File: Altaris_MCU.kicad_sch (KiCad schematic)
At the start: 89 parts, among them J1 Screw_Terminal_01x02, J10 USB_C_Receptacle_USB2.0_16P, J11 Screw_Terminal_01x02, J12 Screw_Terminal_01x02, J13 Screw_Terminal_01x02, J14 Screw_Terminal_01x02, J16 Conn_01x06, J2 Screw_Terminal_01x02, J3 Screw_Terminal_01x02, J4 Screw_Terminal_01x02, J5 Screw_Terminal_01x02, J6 Screw_Terminal_01x02, J7 Conn_01x08_Socket, J8 Screw_Terminal_01x02, J9 USB_C_Receptacle_USB2.0_16P, Q1 Q_NMOS, SW2 RESET1, SW3 BOOT1, U1 ESP32-S3-WROOM-1, U10 USBLC6-2SC6, U11 MAX31855TASA, U12 TPS62827DMQT, U13 USBLC6-2SC6, U15 CH340X, U17 MAX31855TASA, U18 MAX31855TASA, U2 MAX31855KASA, U3 TPS79333-EP, U4 ICM-20948, U5 TPS79318-EP, U6 SN74AVC4T774RSVR, U7 MAX31855KASA, U8 MAX31855KASA, U9 SN74AVC4T774RSVR

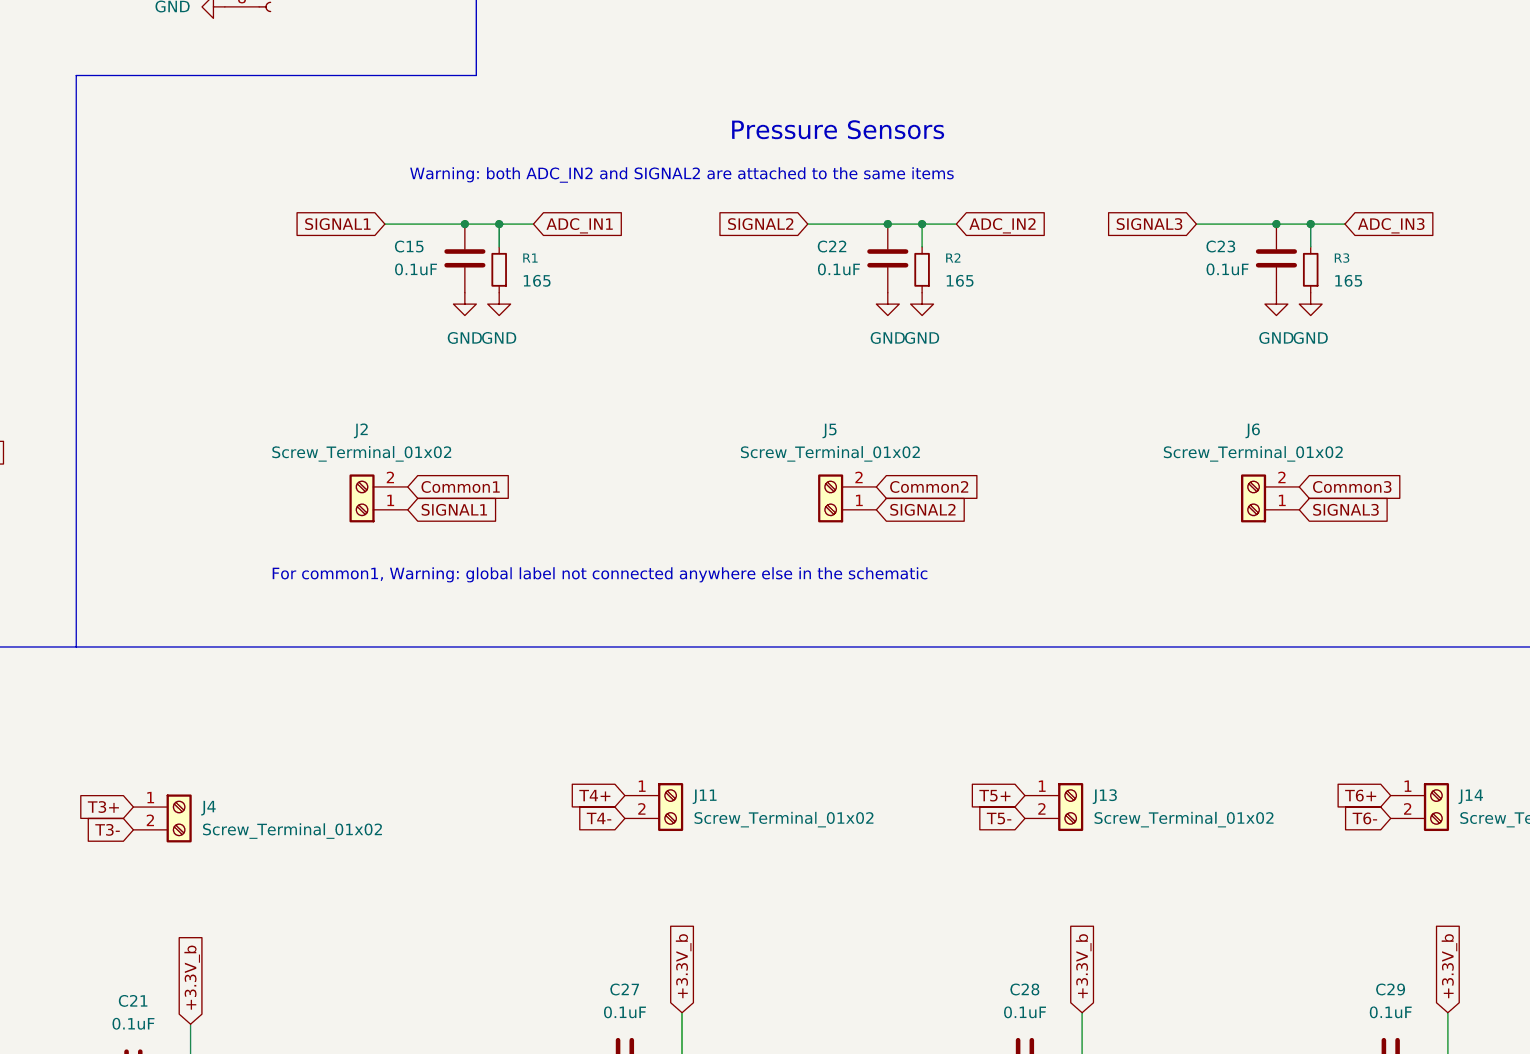
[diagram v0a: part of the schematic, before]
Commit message: minor edits to layout and schematic
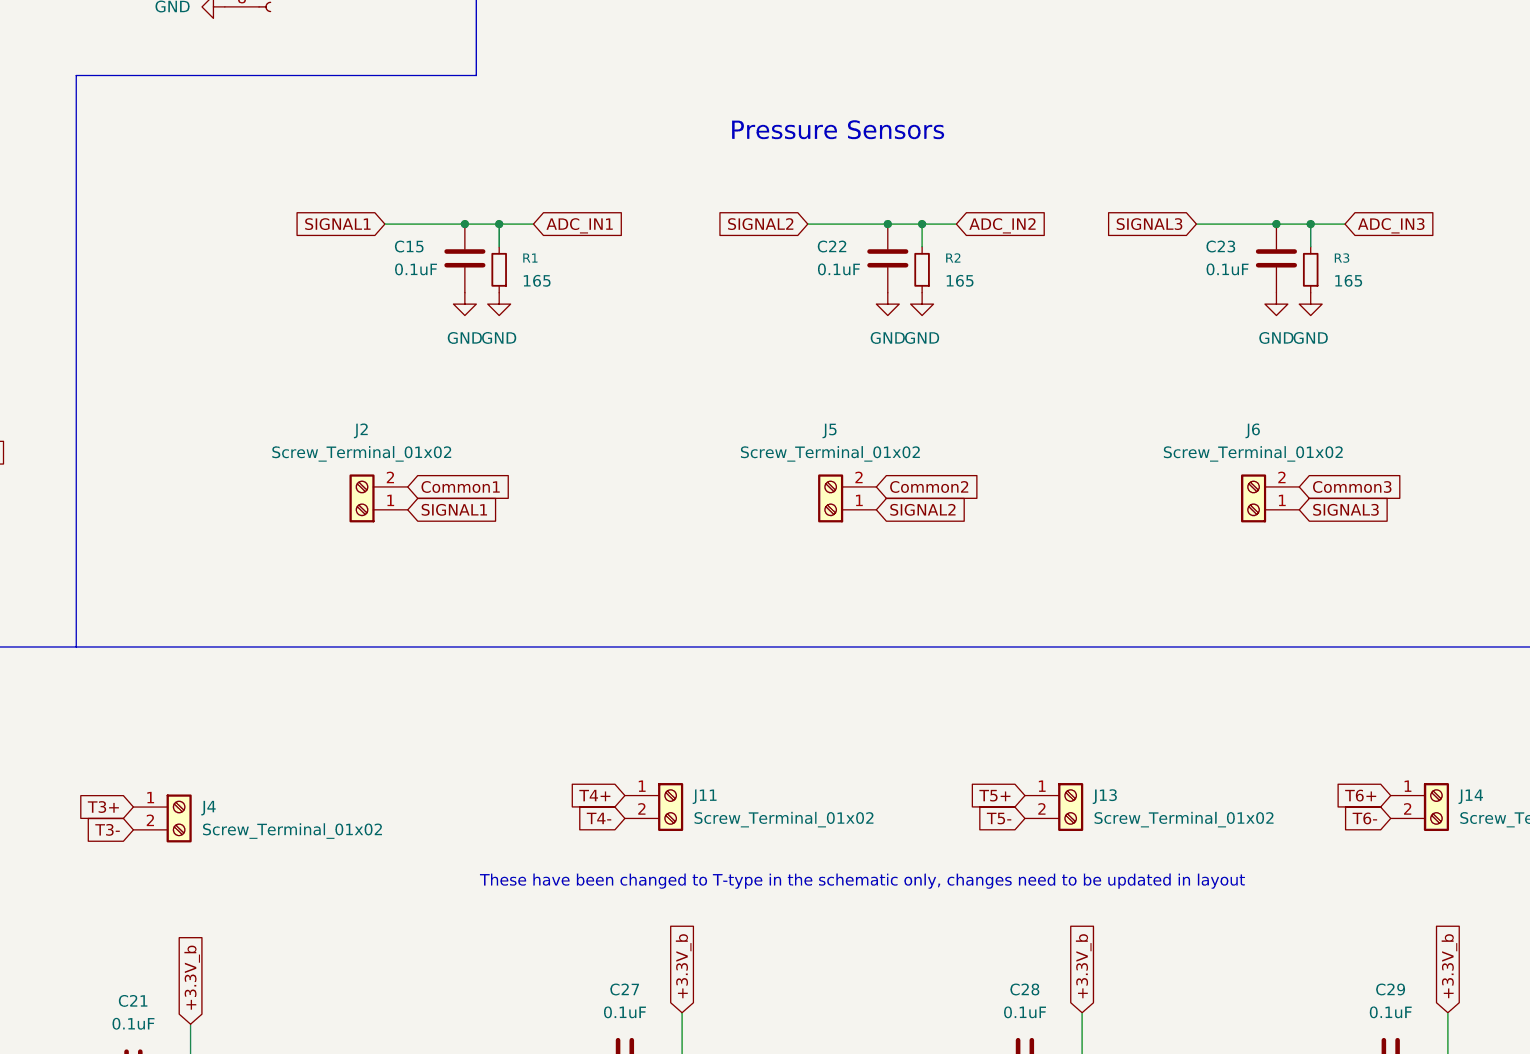
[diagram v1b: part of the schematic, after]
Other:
- note added: "These have been changed to T-type in the schematic only, changes need to be updated in layout"
- note removed: "For common1, Warning: global label not connected anywhere else in the schematic"
- note removed: "Warning: both ADC_IN2 and SIGNAL2 are attached to the same items"
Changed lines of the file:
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@@
+		)
+	)
+	(text "These have been changed to T-type in the schematic only, changes need to be updated in layout\n"
+		(exclude_from_sim no)
+		(at 199.136 140.462 0)
+		(effects
+			(font
+				(size 1.27 1.27)
+			)
 		)
 	)
@@
 		)
 	)
-	(text "For common1, Warning: global label not connected anywhere else in the schematic"
-		(exclude_from_sim no)
-		(at 169.926 106.426 0)
-		(effects
-			(font
-				(size 1.27 1.27)
-			)
-		)
-	)
 	(text "Step-down Converter"
 		(exclude_from_sim no)
@@
 		(effects
 			(font
-				(size 1.27 1.27)
-			)
-		)
-	)
-	(text "Warning: both ADC_IN2 and SIGNAL2 are attached to the same items"
-		(exclude_from_sim no)
-		(at 179.07 61.976 0)
-		(effects
-			(font
